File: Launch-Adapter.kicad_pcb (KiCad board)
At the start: 4 copper layers, 69.6 x 144.5 mm, 85 parts, among them J1 ADC1, J10 +5V_CAN, J11 Input, J2 ADC2, J3 PWM, J4 GPIO, J5 Driver, J6 Measurements, J7 +5V, J8 +15V, J9 +3.3V, U3 ISO1050DUB, U4 ADM3490ExR, U5 LMV324

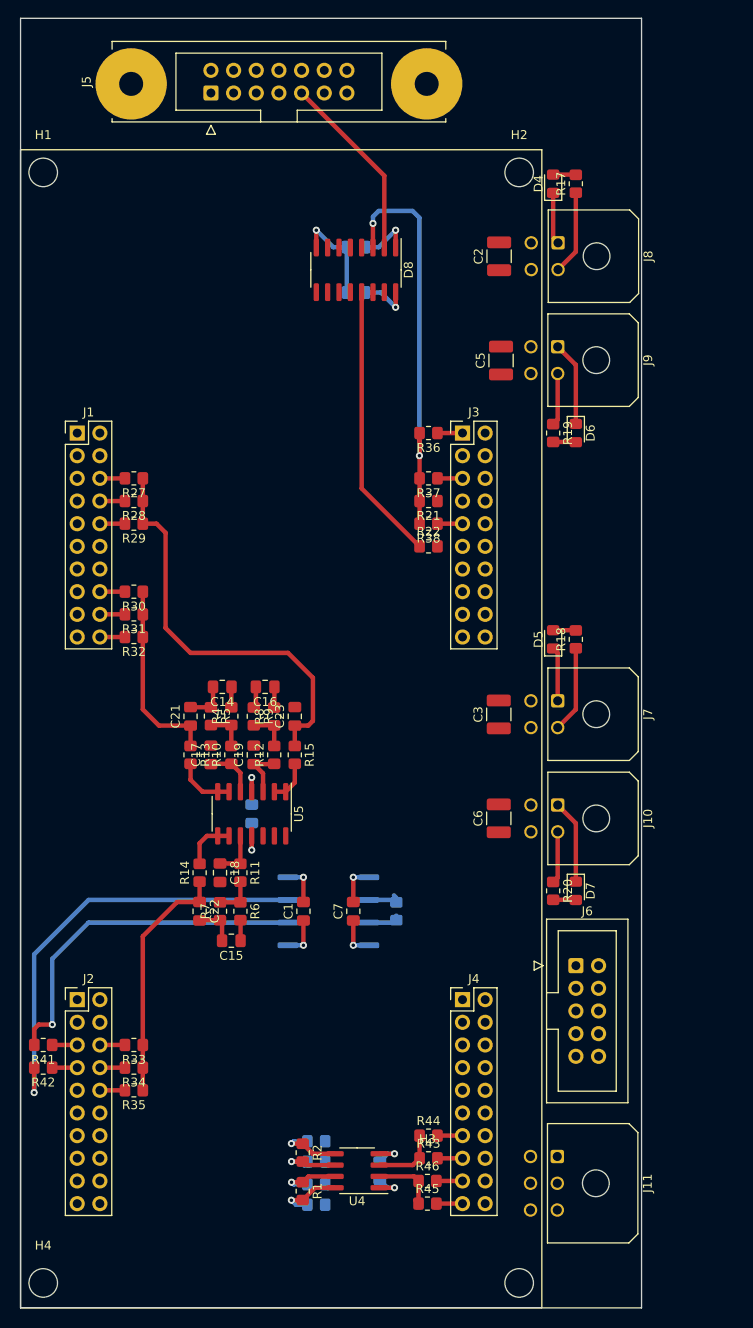
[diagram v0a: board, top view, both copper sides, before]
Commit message: Первая версия в производство
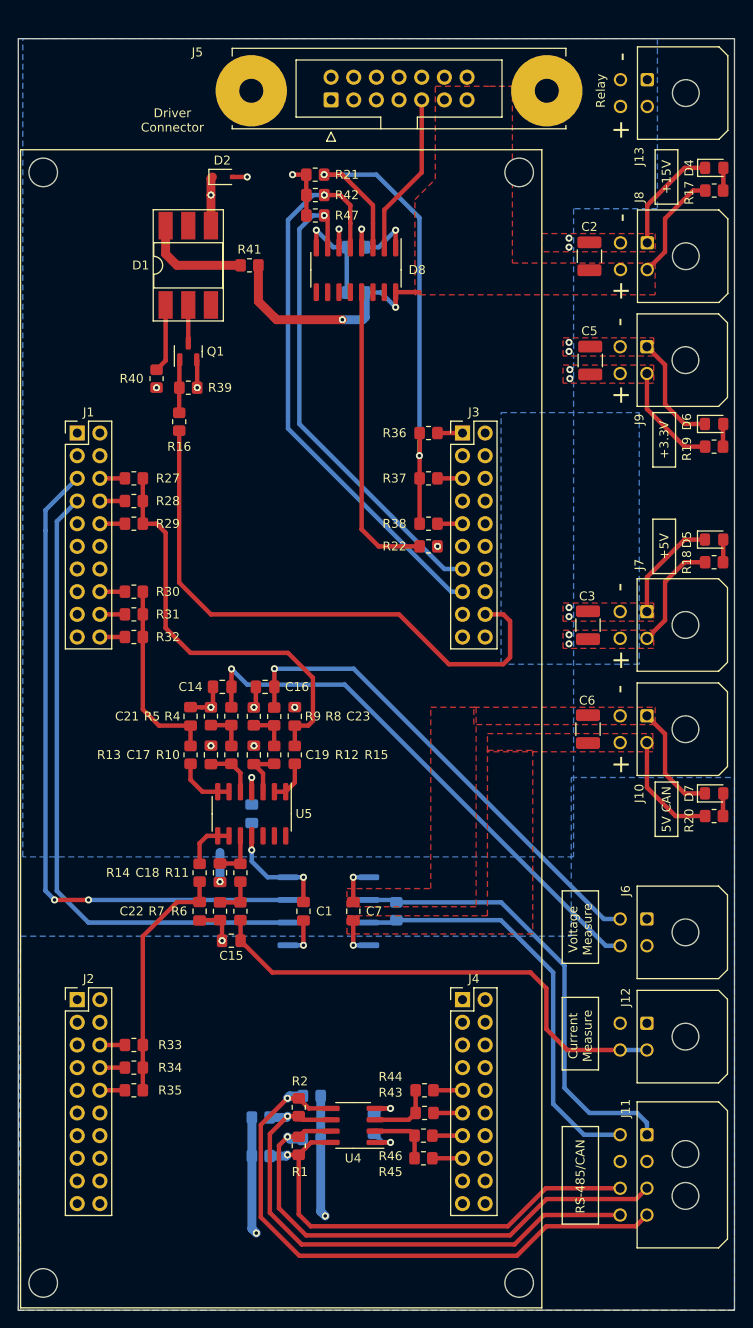
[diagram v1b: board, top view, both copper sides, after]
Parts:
- added D1: PVT412LSPBF, Package_DIP:DIP-6_W8.89mm_SMDSocket_LongPads, F.Cu at (75.4, 45.0)
- added D2: D_Small, Diode_SMD:D_SOD-323F, F.Cu at (79.2, 35.1)
- added J12: Current Measure, Connector_Molex:Molex_Micro-Fit_3.0_43045-0400_2x02_P3.00mm_Horizontal, F.Cu at (126.8, 129.9)
- added J13: Current Measure, Connector_Molex:Molex_Micro-Fit_3.0_43045-0400_2x02_P3.00mm_Horizontal, F.Cu at (126.9, 24.2)
- added Q1: BC817, Package_TO_SOT_SMD:SOT-23, F.Cu at (75.4, 54.6)
- added R16: 4.7k, Resistor_SMD:R_0805_2012Metric_Pad1.20x1.40mm_HandSolder, F.Cu at (74.4, 62.5)
- added R39: 10k, Resistor_SMD:R_0805_2012Metric_Pad1.20x1.40mm_HandSolder, F.Cu at (75.4, 58.7)
- added R40: 220, Resistor_SMD:R_0805_2012Metric_Pad1.20x1.40mm_HandSolder, F.Cu at (71.9, 57.7)
- added R47: 10k, Resistor_SMD:R_0805_2012Metric_Pad1.20x1.40mm_HandSolder, F.Cu at (89.7, 39.4)
- J11: value Input -> Interfaces; footprint Connector_Molex:Molex_Micro-Fit_3.0_43045-0600_2x03_P3.00mm_Horizontal -> Connector_Molex:Molex_Micro-Fit_3.0_43045-0800_2x04_P3.00mm_Horizontal
- J6: value Measurements -> Voltage measure; footprint Connector_IDC:IDC-Header_2x05_P2.54mm_Vertical -> Connector_Molex:Molex_Micro-Fit_3.0_43045-0400_2x02_P3.00mm_Horizontal
- R41: value 0 -> 60
- R42: value 0 -> 10k
- moved R42 102.4 mm to (89.7, 37.1), turned to 0 degrees
- moved R41 90.4 mm to (82.3, 45.0)
- moved R21 38.7 mm to (89.7, 34.8), turned to 0 degrees
- moved D5 21.2 mm to (134.4, 75.7), turned to 0 degrees
- moved R20 19.9 mm to (134.4, 106.7), turned to 0 degrees
- moved D7 19.0 mm to (134.4, 104.1), turned to 0 degrees
- moved D4 18.1 mm to (134.4, 34.0), turned to 0 degrees
- moved R19 18.1 mm to (134.4, 65.3), turned to 0 degrees
- moved R18 17.7 mm to (134.4, 78.2), turned to 0 degrees
- moved R17 15.5 mm to (134.4, 36.6), turned to 0 degrees
- moved D6 15.5 mm to (134.4, 62.7), turned to 0 degrees
- moved C3 14.1 mm to (120.2, 85.3)
- moved C6 14.1 mm to (120.2, 96.9)
- moved J10 14.1 mm to (126.8, 95.4)
- moved J7 14.1 mm to (126.8, 83.8)
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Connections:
- D8 pad 4: unconnected-(D8-Pad4) -> nERR_IN
- D8 pad 5: unconnected-(D8-Pad5) -> nERR_IN_GPIO
- D8 pad 6: unconnected-(D8-Pad6) -> RESET
- D8 pad 7: unconnected-(D8-Pad7) -> RESET_GPIO
- J1 pad 5: unconnected-(J1-Pad5) -> TXD
- J1 pad 7: unconnected-(J1-Pad7) -> RXD
- J11 pad 1: unconnected-(J11-Pad1) -> CANL
- J11 pad 2: unconnected-(J11-Pad2) -> V_IN_PWR
- J11 pad 3: unconnected-(J11-Pad3) -> B
- J11 pad 4: unconnected-(J11-Pad4) -> Y
- J11 pad 5: unconnected-(J11-Pad5) -> CANH
- J11 pad 6: unconnected-(J11-Pad6) -> GNDD
- J2 pad 5: Net-(J2-Pad5) -> unconnected-(J2-Pad5)
- J2 pad 7: Net-(J2-Pad7) -> unconnected-(J2-Pad7)
- J3 pad 13: unconnected-(J3-Pad13) -> RESET_GPIO
- J3 pad 15: unconnected-(J3-Pad15) -> nERR_IN_GPIO
- J3 pad 18: unconnected-(J3-Pad18) -> Relay_Control
- J4 pad 11: unconnected-(J4-Pad11) -> Net-(J4-Pad11)
- J4 pad 17: Net-(J4-Pad17) -> unconnected-(J4-Pad17)
- J4 pad 19: Net-(J4-Pad19) -> unconnected-(J4-Pad19)
- J4 pad 9: unconnected-(J4-Pad9) -> Net-(J4-Pad9)
- J6 pad 1: unconnected-(J6-Pad1) -> GND
- J6 pad 2: unconnected-(J6-Pad2) -> GND
- J6 pad 3: unconnected-(J6-Pad3) -> V_IN
- J6 pad 4: unconnected-(J6-Pad4) -> V_OUT
- R23 pad 1: GND -> GNDD
- R24 pad 1: GND -> GNDD
- R41 pad 1: Net-(J2-Pad5) -> +15V
- R41 pad 2: RXD -> Net-(D1-Pad6)
- R42 pad 1: Net-(J2-Pad7) -> GND
- R42 pad 2: TXD -> nERR_IN_GPIO
- R43 pad 2: Net-(J4-Pad15) -> Net-(J4-Pad11)
- R44 pad 2: Net-(J4-Pad13) -> Net-(J4-Pad9)
- R45 pad 2: Net-(J4-Pad19) -> Net-(J4-Pad15)
- R46 pad 2: Net-(J4-Pad17) -> Net-(J4-Pad13)
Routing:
- net V_IN_PWR: track 0.00 -> 67.9 mm, vias 0 -> 1
- net Relay_Control: track 0.00 -> 65.4 mm
- net nERR_IN_GPIO: track 0.00 -> 63.9 mm, vias 0 -> 1
- net Y: track 7.26 -> 68.7 mm
- net V_OUT: track 2.29 -> 60.7 mm, vias 0 -> 1
- net RESET_GPIO: track 0.00 -> 54.0 mm, vias 0 -> 1
- net Z: track 6.85 -> 60.8 mm
- net I_INDUCT: track 2.31 -> 55.6 mm
- net B: track 7.02 -> 60.0 mm
- net V_IN: track 2.33 -> 54.7 mm, vias 0 -> 1
- net GNDD: track 0.00 -> 49.4 mm, vias 0 -> 1
- net CANL: track 3.21 -> 50.5 mm
- net A: track 7.47 -> 52.5 mm
- net CANH: track 3.21 -> 46.5 mm
- net GND: track 57.3 -> 93.5 mm, vias 4 -> 20
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- added copper zone on F.Cu, net +15V
- added copper zone on F.Cu, net +3V3
- added copper zone on In1.Cu, net +3V3
- added copper zone on F.Cu, net +5V
- added copper zone on In2.Cu, net +5V
- added copper zone on F.Cu, net +5VD
- added copper zone on B.Cu, net GND
- added copper zone on F.Cu, net GND
- added copper zone on F.Cu, net GND2
- added copper zone on In1.Cu, net Net-(D1-Pad4)
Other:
- board size 69.6 x 144.5 mm -> 80.3 x 142.5 mm
- board text added: "+"
- board text added: "+15V"
- board text added: "+3.3V"
- board text added: "+5V"
- board text added: "-"
- board text added: "5V CAN"
- board text added: "Current Measure"
- board text added: "Driver Connector"
- board text added: "RS-485/CAN"
- board text added: "Relay"
- board text added: "Voltage Measure"
